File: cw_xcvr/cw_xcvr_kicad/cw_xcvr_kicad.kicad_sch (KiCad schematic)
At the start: 0 parts

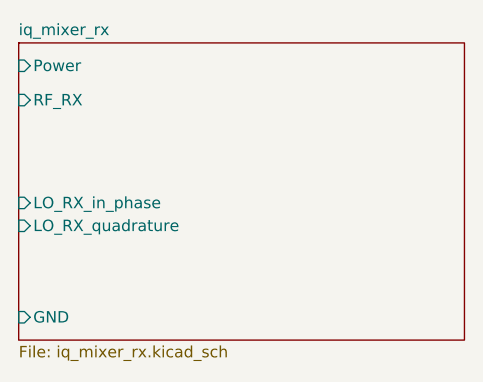
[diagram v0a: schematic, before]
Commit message: Rx work
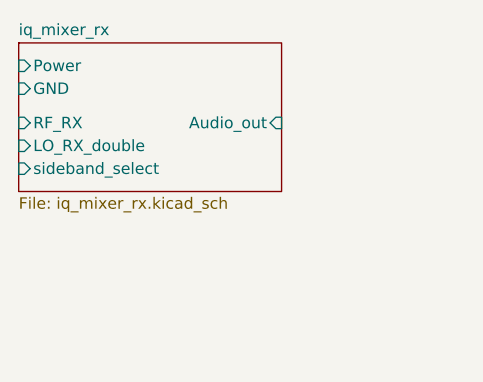
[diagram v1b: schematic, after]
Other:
- sheet iq_mixer_rx ports: added Audio_out, LO_RX_double, sideband_select; removed LO_RX_in_phase, LO_RX_quadrature
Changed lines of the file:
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@@
 	(sheet
 		(at 198.12 26.67)
-		(size 49.53 33.02)
+		(size 29.21 16.51)
 		(exclude_from_sim no)
 		(in_bom yes)
@@
 		)
 		(property "Sheetfile" "iq_mixer_rx.kicad_sch"
-			(at 198.12 60.2746 0)
+			(at 198.12 43.7646 0)
 			(effects
 				(font
@@
 		)
 		(pin "GND" input
-			(at 198.12 57.15 180)
-			(effects
-				(font
-					(size 1.27 1.27)
-				)
-				(justify left)
-			)
-		)
-		(pin "LO_RX_in_phase" input
-			(at 198.12 44.45 180)
-			(effects
-				(font
-					(size 1.27 1.27)
-				)
-				(justify left)
-			)
-		)
-		(pin "LO_RX_quadrature" input
-			(at 198.12 46.99 180)
+			(at 198.12 31.75 180)
 			(effects
 				(font
@@
 		)
 		(pin "RF_RX" input
-			(at 198.12 33.02 180)
+			(at 198.12 35.56 180)
 			(effects
 				(font
+					(size 1.27 1.27)
+				)
+				(justify left)
+			)
+		)
+		(pin "Audio_out" input
+			(at 227.33 35.56 0)
+			(effects
+				(font
+					(size 1.27 1.27)
+				)
+				(justify right)
+			)
+		)
+		(pin "LO_RX_double" input
+			(at 198.12 38.1 180)
+			(effects
+				(font
+					(size 1.27 1.27)
+				)
+				(justify left)
+			)
+		)
+		(pin "sideband_select" input
+			(at 198.12 40.64 180)
+			(effects
+				(font
